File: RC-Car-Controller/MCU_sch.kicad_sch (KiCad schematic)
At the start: 16 parts, among them SW1 SW_Push, U7 STM32H743VGTx, Y1 Crystal

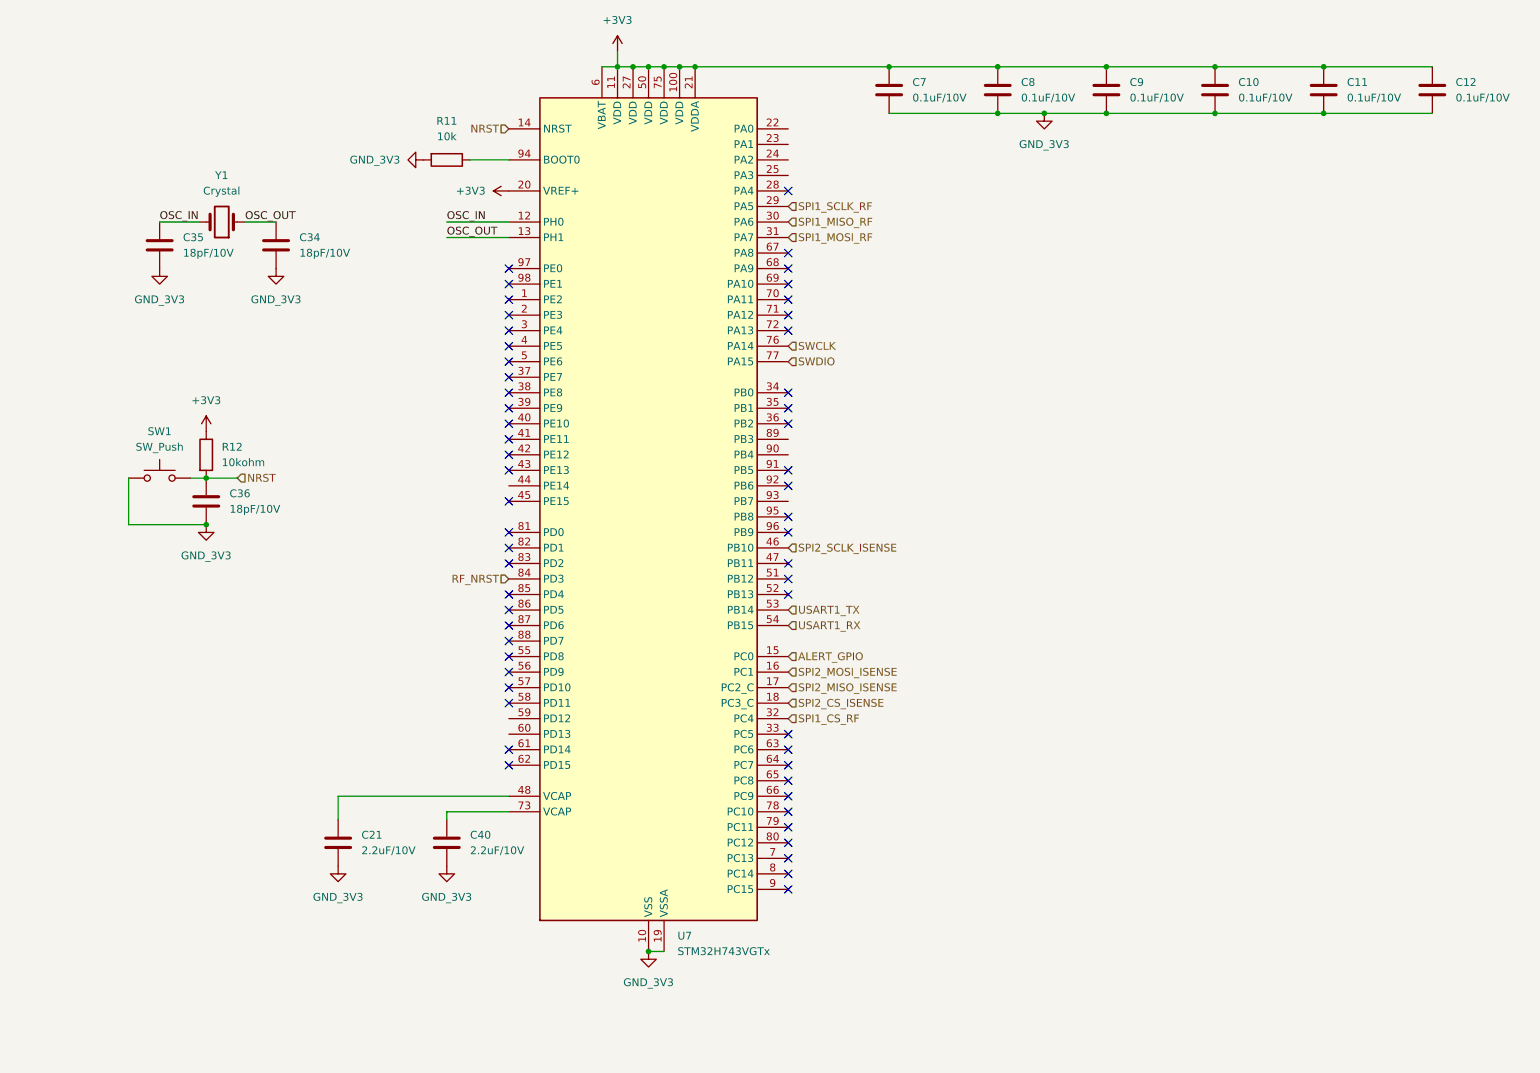
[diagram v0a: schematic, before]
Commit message: Finished prelim. Controller
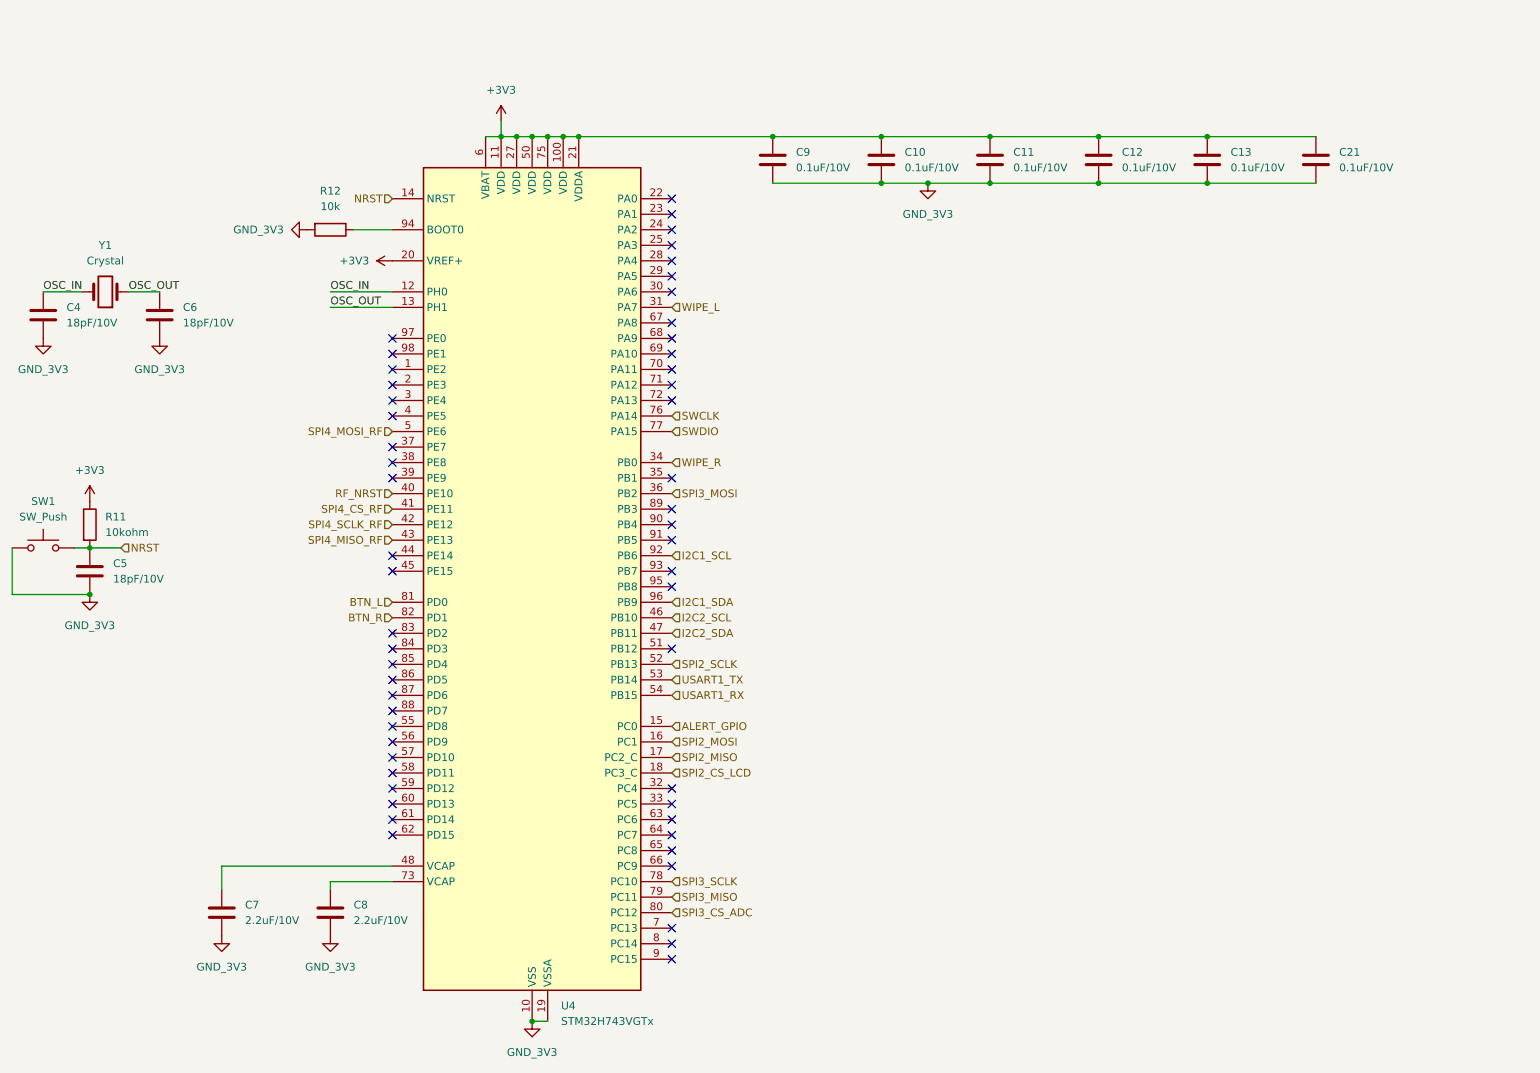
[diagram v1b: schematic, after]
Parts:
- removed C34, C35, C36: 18pF/10V, Capacitor_SMD:C_0201_0603Metric, symbol Device:C
- removed C40: 2.2uF/10V, Capacitor_SMD:C_0201_0603Metric, symbol Device:C
- removed U7: STM32H743VGTx, Package_QFP:LQFP-100_14x14mm_P0.5mm, symbol MCU_ST_STM32H7:STM32H743VGTx
- added C13: 0.1uF/10V, Capacitor_SMD:C_0201_0603Metric, symbol Device:C
- added C4, C5, C6: 18pF/10V, Capacitor_SMD:C_0201_0603Metric, symbol Device:C
- added U4: STM32H743VGTx, Package_QFP:LQFP-100_14x14mm_P0.5mm, symbol MCU_ST_STM32H7:STM32H743VGTx
- C21: value 2.2uF/10V -> 0.1uF/10V
- C7, C8: value 0.1uF/10V -> 2.2uF/10V
- R11: value 10k -> 10kohm
- R12: value 10kohm -> 10k
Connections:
- net +3V3: now also C21.1, R11.1, C13.1, U4.100 (VDD), U4.11 (VDD), U4.20 (VREF+), U4.21 (VDDA), U4.27 (VDD), U4.50 (VDD), U4.6 (VBAT), U4.75 (VDD); no longer C7.1, C8.1, R12.1
- net ALERT_GPIO: now also U4.15 (PC0)
- net GND_3V3: now also R12.2, C13.2, C4.2, C5.2, C6.2, U4.10 (VSS), U4.19 (VSSA), U4.26 (VSS), U4.49 (VSS), U4.74 (VSS), U4.99 (VSS); no longer R11.2
- net NRST: now also R11.2, C5.1, U4.14 (NRST); no longer R12.2
- net OSC_IN: now also C4.1, U4.12 (PH0)
- net OSC_OUT: now also C6.1, U4.13 (PH1)
- net RF_NRST: now also U4.40 (PE10)
- net SWCLK: now also U4.76 (PA14)
- net SWDIO: now also U4.77 (PA15)
- net USART1_RX: now also U4.54 (PB15)
- net USART1_TX: now also U4.53 (PB14)
- new net: R12.1, U4.94 (BOOT0)
- new net: C7.1, U4.48 (VCAP)
- new net: C8.1, U4.73 (VCAP)
- new net BTN_L: U4.81 (PD0)
- new net BTN_R: U4.82 (PD1)
- new net I2C1_SCL: U4.92 (PB6)
- new net I2C1_SDA: U4.96 (PB9)
- new net I2C2_SCL: U4.46 (PB10)
- new net I2C2_SDA: U4.47 (PB11)
- new net SPI2_CS_LCD: U4.18 (PC3_C)
- new net SPI2_MISO: U4.17 (PC2_C)
- new net SPI2_MOSI: U4.16 (PC1)
- new net SPI2_SCLK: U4.52 (PB13)
- new net SPI3_CS_ADC: U4.80 (PC12)
- new net SPI3_MISO: U4.79 (PC11)
- new net SPI3_MOSI: U4.36 (PB2)
- new net SPI3_SCLK: U4.78 (PC10)
- new net SPI4_CS_RF: U4.41 (PE11)
- new net SPI4_MISO_RF: U4.43 (PE13)
- new net SPI4_MOSI_RF: U4.5 (PE6)
- new net SPI4_SCLK_RF: U4.42 (PE12)
- new net WIPE_L: U4.31 (PA7)
- new net WIPE_R: U4.34 (PB0)
- no-connect marks 56 -> 54
